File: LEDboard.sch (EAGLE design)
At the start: 304 parts, among them IC1 REG1117, U1 IS31FL3741_QFN60, U2 IS31FL3741_QFN60, U4 TPS61090RSAR, U5 MCP73831T-2ACI/OT, Y1 32.768kHz

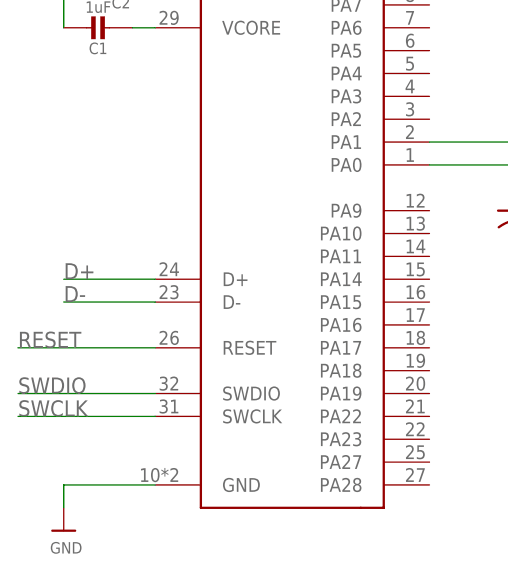
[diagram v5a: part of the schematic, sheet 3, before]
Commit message: diff pair
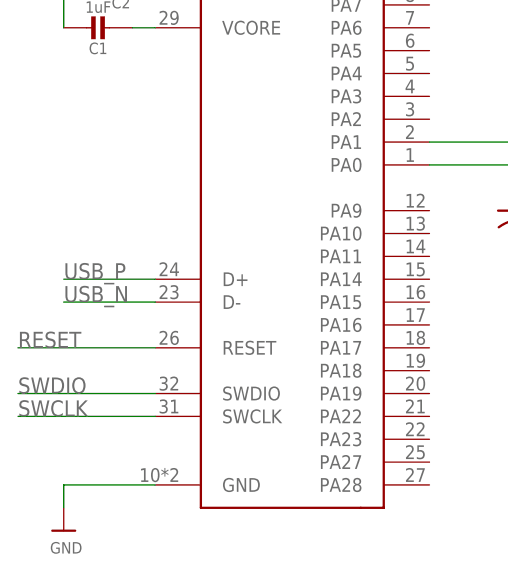
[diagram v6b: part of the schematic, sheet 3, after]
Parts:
- renumbered MCU to U3
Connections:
- net D+ renamed USB_P
- net D- renamed USB_N
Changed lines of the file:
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@@
 <class number="0" name="default" width="0" drill="0">
 </class>
+<class number="1" name="diff_pairs" width="0.254" drill="0">
+</class>
 </classes>
 <parts>
@@
 <part name="U$12" library="microbuilder" deviceset="5.0V" device=""/>
 <part name="U$13" library="microbuilder" deviceset="5.0V" device="" value="3V3"/>
-<part name="MCU" library="adafruit" deviceset="ATSAMD21E" device=""/>
+<part name="U3" library="adafruit" deviceset="ATSAMD21E" device=""/>
 <part name="U$6" library="microbuilder" deviceset="5.0V" device="" value="3V3"/>
 <part name="C1" library="microbuilder" deviceset="CAP_CERAMIC" device="0805-NOOUTLINE" value="1uF"/>
@@
 </plain>
 <instances>
-<instance part="MCU" gate="G$1" x="50.8" y="48.26"/>
+<instance part="U3" gate="G$1" x="50.8" y="48.26"/>
 <instance part="U$6" gate="G$1" x="22.86" y="81.28"/>
 <instance part="C1" gate="G$1" x="27.94" y="66.04" rot="R90"/>
@@
 </busses>
 <nets>
-<net name="D-" class="0">
+<net name="USB_N" class="1">
 <segment>
-<pinref part="MCU" gate="G$1" pin="D-"/>
+<pinref part="U3" gate="G$1" pin="D-"/>
 <wire x1="33.02" y1="35.56" x2="22.86" y2="35.56" width="0.1524" layer="91"/>
 <label x="22.86" y="35.56" size="1.778" layer="95"/>
 </segment>
 </net>
-<net name="D+" class="0">
+<net name="USB_P" class="1">
 <segment>
-<pinref part="MCU" gate="G$1" pin="D+"/>
+<pinref part="U3" gate="G$1" pin="D+"/>
 <wire x1="33.02" y1="38.1" x2="22.86" y2="38.1" width="0.1524" layer="91"/>
 <label x="22.86" y="38.1" size="1.778" layer="95"/>
@@
 <net name="N$75" class="0">
 <segment>
-<pinref part="MCU" gate="G$1" pin="VCORE"/>
+<pinref part="U3" gate="G$1" pin="VCORE"/>
 <pinref part="C1" gate="G$1" pin="2"/>
 <wire x1="33.02" y1="66.04" x2="30.48" y2="66.04" width="0.1524" layer="91"/>
@@
 <wire x1="22.86" y1="15.24" x2="22.86" y2="12.7" width="0.1524" layer="91"/>
 <pinref part="U$9" gate="G$1" pin="GND"/>
-<pinref part="MCU" gate="G$1" pin="GND"/>
+<pinref part="U3" gate="G$1" pin="GND"/>
 <wire x1="33.02" y1="15.24" x2="22.86" y2="15.24" width="0.1524" layer="91"/>
 </segment>
@@
 <segment>
 <pinref part="C2" gate="G$1" pin="2"/>
-<pinref part="MCU" gate="G$1" pin="VDD"/>
+<pinref part="U3" gate="G$1" pin="VDD"/>
 </segment>
 </net>
 <net name="N$78" class="0">
 <segment>
-<pinref part="MCU" gate="G$1" pin="PA1"/>
+<pinref part="U3" gate="G$1" pin="PA1"/>
 <wire x1="63.5" y1="53.34" x2="81.28" y2="53.34" width="0.1524" layer="91"/>
 <pinref part="Y1" gate="G$1" pin="1"/>
@@
 <net name="N$79" class="0">
 <segment>
-<pinref part="MCU" gate="G$1" pin="PA0"/>
+<pinref part="U3" gate="G$1" pin="PA0"/>
 <pinref part="Y1" gate="G$1" pin="2"/>
 <wire x1="63.5" y1="50.8" x2="73.66" y2="50.8" width="0.1524" layer="91"/>
@@
 <net name="RESET" class="0">
 <segment>
-<pinref part="MCU" gate="G$1" pin="RESET"/>
+<pinref part="U3" gate="G$1" pin="RESET"/>
 <wire x1="33.02" y1="30.48" x2="17.78" y2="30.48" width="0.1524" layer="91"/>
 <label x="17.78" y="30.48" size="1.778" layer="95"/>
@@
 <net name="SWDIO" class="0">
 <segment>
-<pinref part="MCU" gate="G$1" pin="SWDIO"/>
+<pinref part="U3" gate="G$1" pin="SWDIO"/>
 <wire x1="33.02" y1="25.4" x2="17.78" y2="25.4" width="0.1524" layer="91"/>
 <label x="17.78" y="25.4" size="1.778" layer="95"/>
@@
 <net name="SWCLK" class="0">
 <segment>
-<pinref part="MCU" gate="G$1" pin="SWCLK"/>
+<pinref part="U3" gate="G$1" pin="SWCLK"/>
 <wire x1="33.02" y1="22.86" x2="17.78" y2="22.86" width="0.1524" layer="91"/>
 <label x="17.78" y="22.86" size="1.778" layer="95"/>
@@
 </segment>
 </net>
-<net name="D-" class="0">
+<net name="USB_N" class="1">
 <segment>
 <pinref part="J2" gate="G$1" pin="D-"/>
@@
 </segment>
 </net>
-<net name="D+" class="0">
+<net name="USB_P" class="1">
 <segment>
 <pinref part="J2" gate="G$1" pin="D+"/>
